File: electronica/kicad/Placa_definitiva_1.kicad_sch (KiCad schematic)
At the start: 24 parts, among them J1 conec., J2 conec., J3 conec., J4 conec., J5 conec., Q1 Q_NPN, U1 ESP32-C3-DevKitM-1

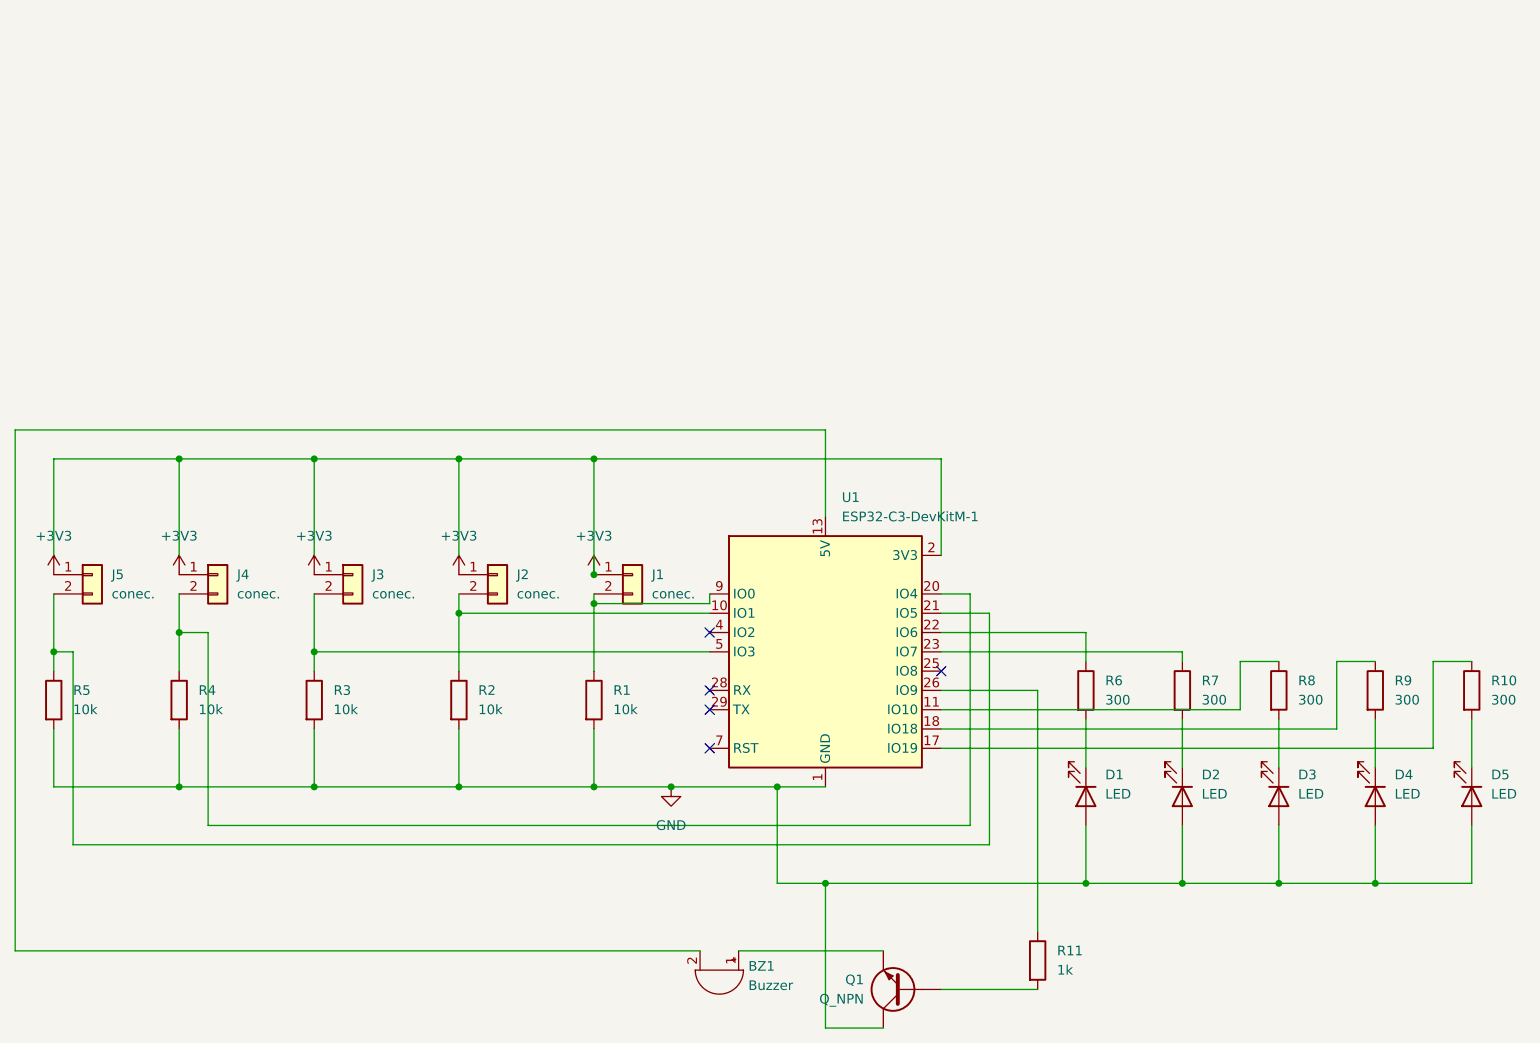
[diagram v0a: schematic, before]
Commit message: Add files via upload
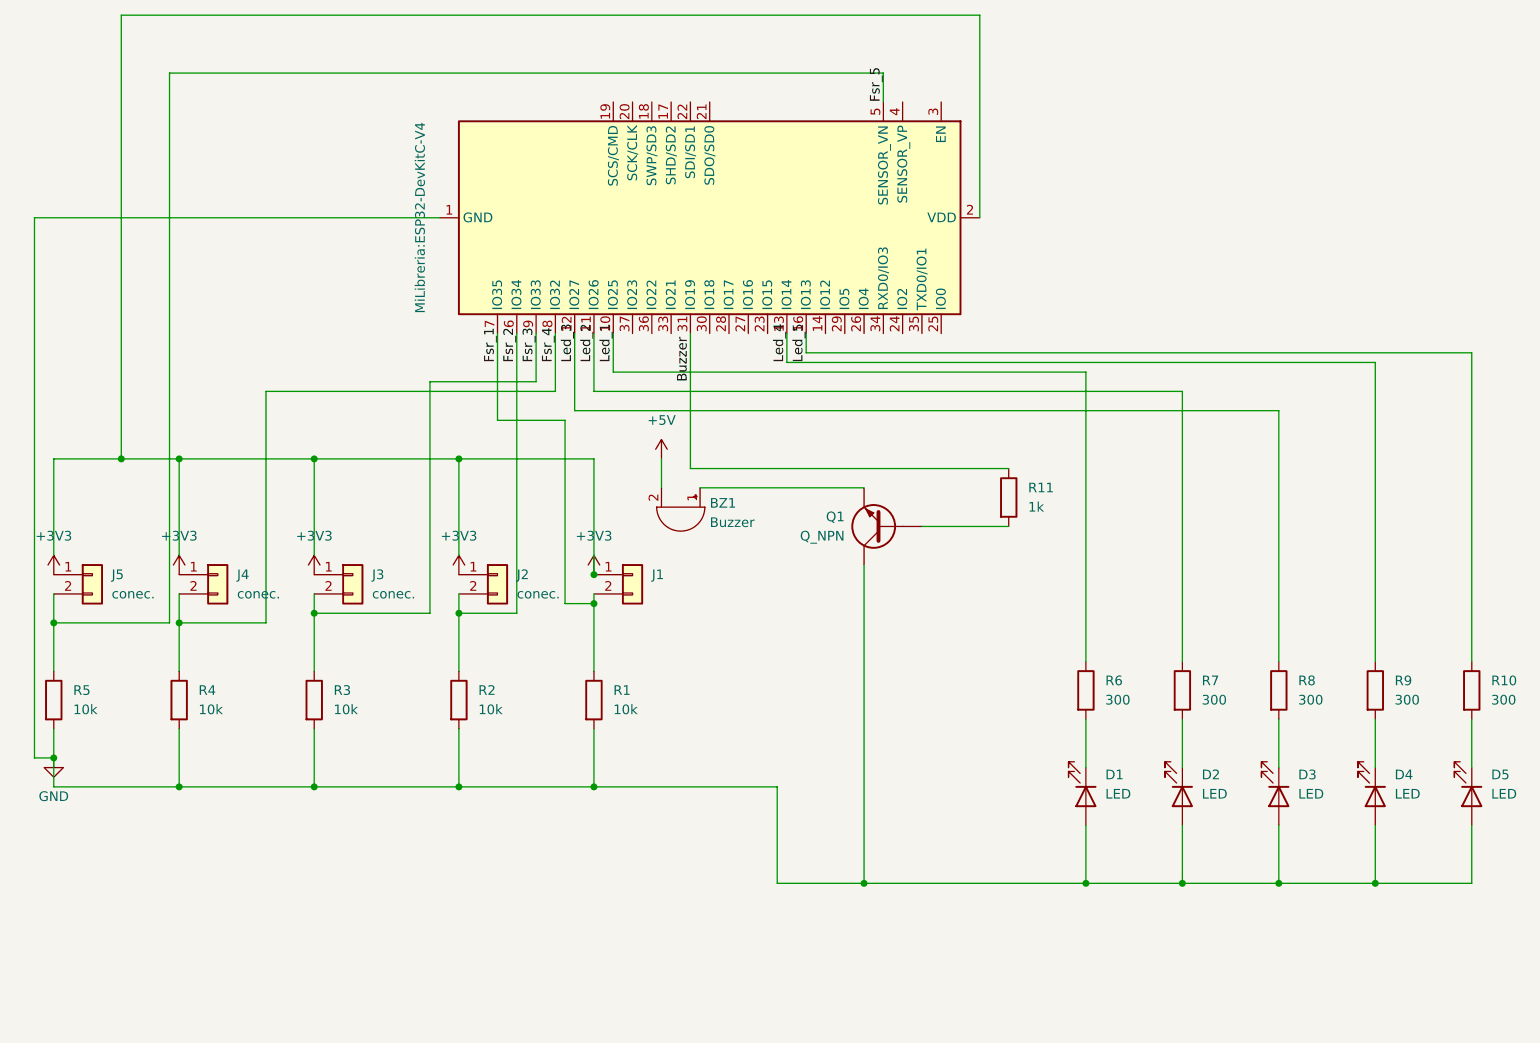
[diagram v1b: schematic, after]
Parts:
- removed U1: ESP32-C3-DevKitM-1, RF_Module:ESP32-C3-DevKitM-1, symbol RF_Module:ESP32-C3-DevKitM-1
- added U1: ESP32-WROOM-32, MiLibreria:ESP32-DevKitC-V4, symbol RF_Module:ESP32-WROOM-32
- BZ1: footprint (none) -> Buzzer_Beeper:Buzzer_12x9.5RM7.6
- D1, D2, D3, D4, D5: footprint (none) -> LED_THT:LED_D5.0mm
- J1, J2, J3, J4, J5: footprint RF_Module:ESP32-C3-DevKitM-1 -> Connector_PinHeader_2.54mm:PinHeader_1x02_P2.54mm_Vertical
- Q1: footprint (none) -> Package_TO_SOT_THT:TO-92_Inline
- R1, R10, R11, R2, R3, R4, R5, R6, R7, R8, R9: footprint (none) -> Resistor_THT:R_Axial_DIN0207_L6.3mm_D2.5mm_P10.16mm_Horizontal
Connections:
- net +3V3: now also U1.2 (VDD)
- net GND: now also U1.1 (GND), U1.15 (GND), U1.38 (GND), U1.39 (GND)
- net Fsr_2: now reaches J2.2 (Pin_2), R2.1
- net Fsr_2: now also U1.6 (IO34)
- net Led_3: now reaches R8.1
- net Led_3: now also U1.12 (IO27)
- net +5V: now reaches BZ1.2 (-)
- net at R10.1: now also U1.16 (IO13)
- net Led_4: now reaches R9.1
- net Led_4: now also U1.13 (IO14)
- net Fsr_4: now reaches J4.2 (Pin_2), R4.1
- net Fsr_4: now also U1.8 (IO32)
- net Fsr_5: now reaches J5.2 (Pin_2), R5.1
- net Fsr_5: now also U1.5 (SENSOR_VN)
- net Led_1: now reaches R6.1
- net Led_1: now also U1.10 (IO25)
- net Led_2: now reaches R7.1
- net Led_2: now also U1.11 (IO26)
- net Buzzer: now reaches R11.1
- net Buzzer: now also U1.31 (IO19)
- net Fsr_3: now reaches J3.2 (Pin_2), R3.1
- net Fsr_3: now also U1.9 (IO33)
- net Fsr_1: now reaches J1.2 (Pin_2), R1.1
- net Fsr_1: now also U1.7 (IO35)
- no-connect marks 5 -> 0
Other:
- moved on the sheet: BZ1, Q1, R11
